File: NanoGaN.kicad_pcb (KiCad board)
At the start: 6 copper layers, 54 x 94 mm, 222 parts, among them J1 U_DC, J10 Conn_01x06, J11 Conn_01x04, J12 USB4085-GF-A, J14 Conn_01x03, J2 GND, J3 Phase_U, J4 Phase_V, J5 Phase_W, J6 FTSH-107-01-L-DV-K-TR, J7 Conn_01x03, J8 Conn_01x02, J9 Conn_01x07, Q1 IGC025S08S1, Q2 IGC025S08S1, Q3 IGC025S08S1, Q4 IGC025S08S1, Q5 IGC025S08S1, Q6 IGC025S08S1, Q7 Si2302CDS, U1 STM32H723VGTx, U10 SN74LVC1G66DCKR, U11 SN74LVC1G66DCKR, U12 LMG1205YFXR, U13 BMI323, U14 AS5047P-ATST, U15 TCAN1044VDRQ1, U16 SN74LVC1G66DCKR, U17 AD8418, U18 SN74LVC1G66DCKR, U19 NCS2220AMUT1G, U2 LMR51635XDDCR, U20 NCS2220AMUT1G, U21 NCS2220AMUT1G, U3 AMS1117, U4 AD8418, U5 LMG1205YFXR, U6 SN74LVC1G66DCKR, U7 SN74LVC1G66DCKR, U8 LMG1205YFXR, U9 AD8418, X1 8MHz

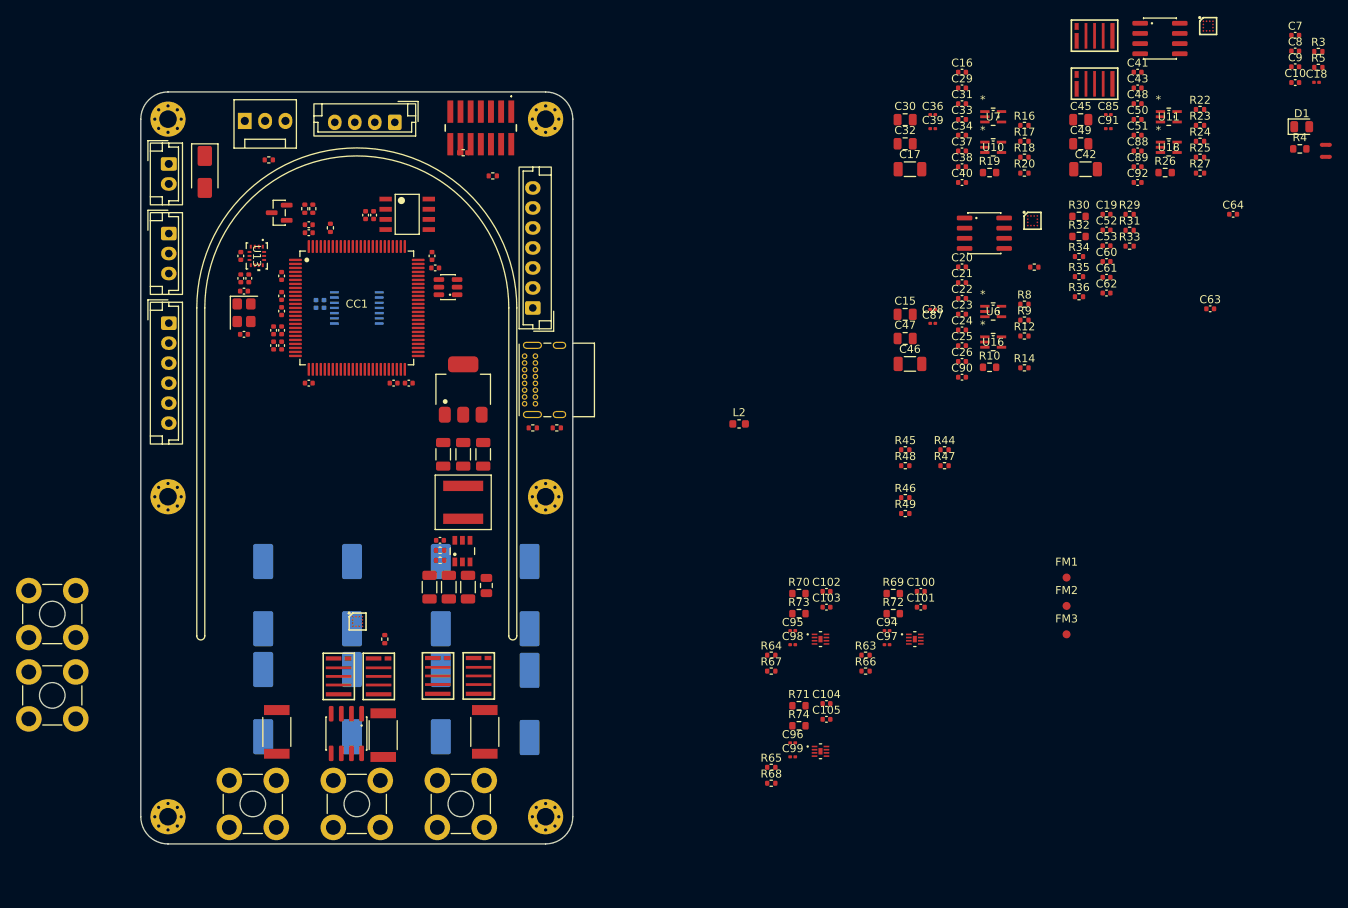
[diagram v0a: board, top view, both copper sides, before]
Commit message: added the first draft of the layout
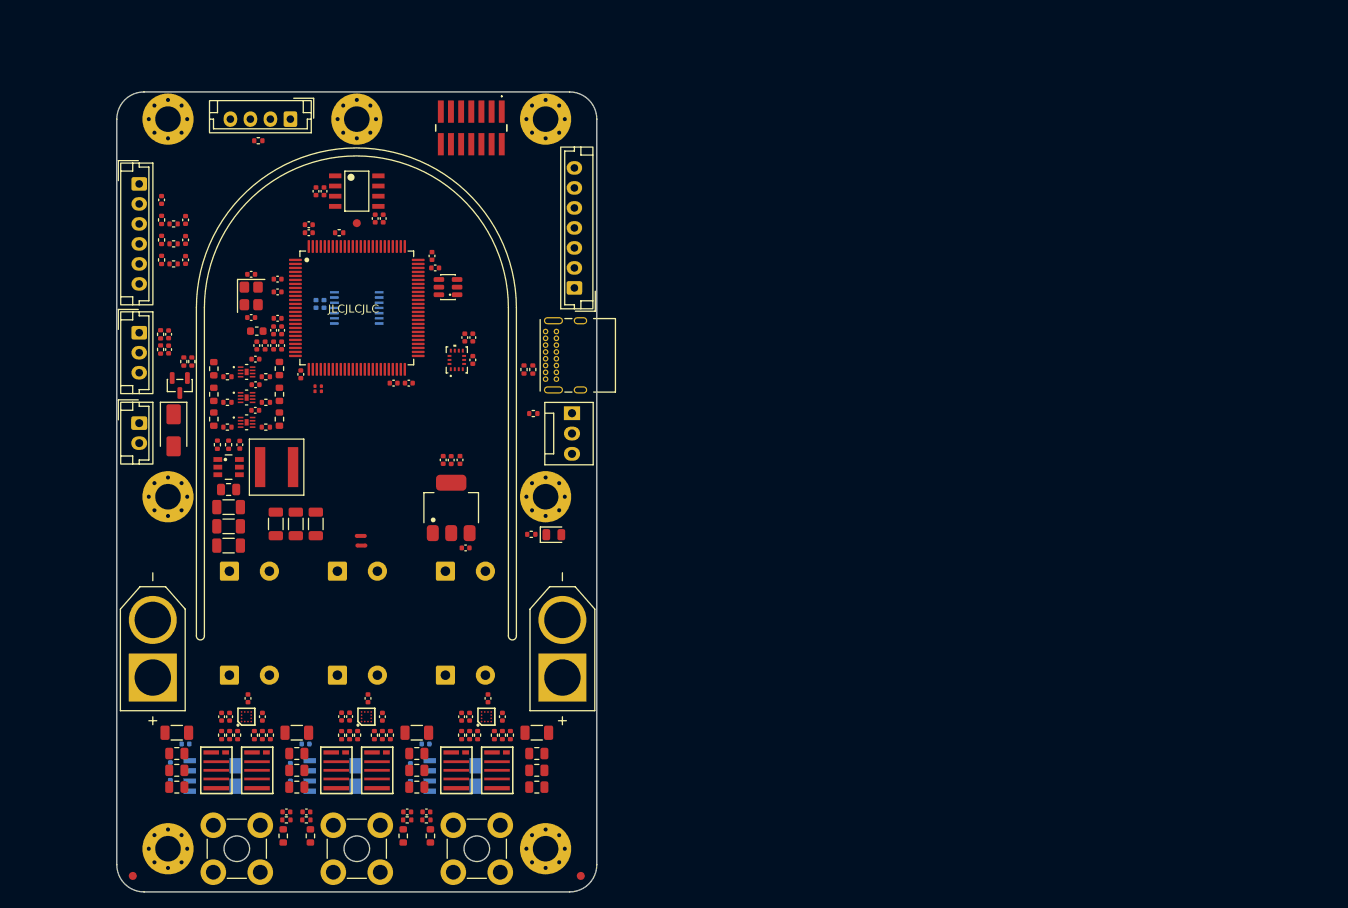
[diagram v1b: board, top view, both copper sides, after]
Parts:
- removed C102, C104: 1u, Capacitor_SMD:C_0402_1005Metric
- removed C103, C105: 100n, Capacitor_SMD:C_0402_1005Metric
- removed C96, C97, C98, C99: 1n, Capacitor_SMD:C_0201_0603Metric
- removed R28: 1m, NanoGaN:RES_00FEA_VIS-L
- removed R30, R32: 10k, Resistor_SMD:R_0603_1608Metric
- removed R7: 10k, Resistor_SMD:R_0402_1005Metric
- removed U10, U11, U16, U18: SN74LVC1G66DCKR, NanoGaN:DCK5
- removed U17, U9: AD8418, Package_SO:SOIC-8_3.9x4.9mm_P1.27mm
- added C67: 100n, Capacitor_SMD:C_0805_2012Metric, F.Cu at (152.7, 134.9)
- added C68: 1u, Capacitor_SMD:C_1206_3216Metric, F.Cu at (167.7, 128.1)
- added MH7: M3, MountingHole:MountingHole_3.2mm_M3_Pad_Via, F.Cu at (168.8, 142.6)
- C100: value 1u -> 100n
- C11, C12, C13, C14, C27, C35: value 150u -> 470u; footprint Capacitor_SMD:CP_Elec_10x10.5 -> Capacitor_THT:CP_Radial_D12.5mm_P5.00mm
- C18, C36, C85, C87: footprint Capacitor_SMD:C_0201_0603Metric -> Capacitor_SMD:C_0402_1005Metric
- C24, C25, C33, C38, C89: moved to B.Cu
- C26: value 1u -> 100n; moved to B.Cu
- C28, C39, C91: value 1n -> 100p; footprint Capacitor_SMD:C_0201_0603Metric -> Capacitor_SMD:C_0402_1005Metric; moved to B.Cu
- C37: value 1u -> 4u7
- C40: value 15n -> 4u7
- C44, C81: value 150u -> 100n; footprint Capacitor_SMD:CP_Elec_10x10.5 -> Capacitor_SMD:C_0805_2012Metric; moved to F.Cu
- C50: footprint Capacitor_SMD:C_0402_1005Metric -> Capacitor_SMD:C_0805_2012Metric
- C88: value 1u -> 100n; footprint Capacitor_SMD:C_0402_1005Metric -> Capacitor_SMD:C_0805_2012Metric
- C90: value 15n -> 100n; footprint Capacitor_SMD:C_0402_1005Metric -> Capacitor_SMD:C_0805_2012Metric
- C92: value 15n -> 100n
- J1: value U_DC -> XT60-M; footprint TerminalBlock_Wuerth:Wuerth_REDCUBE-THR_WP-THRBU_74650073_THR -> NanoGaN:AMASS_XT60-M
- J2: value GND -> XT60-M; footprint TerminalBlock_Wuerth:Wuerth_REDCUBE-THR_WP-THRBU_74650073_THR -> NanoGaN:AMASS_XT60-M
- MH1, MH2, MH3, MH4, MH5, MH6: value M2 -> M3; footprint MountingHole:MountingHole_2.2mm_M2_Pad_Via -> MountingHole:MountingHole_3.2mm_M3_Pad_Via
- R11, R21: value 1m -> 10k; footprint NanoGaN:RES_00FEA_VIS-L -> Resistor_SMD:R_0402_1005Metric
- U4: value AD8418 -> ACS37030LLZATR-065B3; footprint Package_SO:SOIC-8_3.9x4.9mm_P1.27mm -> NanoGaN:ACS37030LLZATR020B3; moved to B.Cu
- U6, U7: value SN74LVC1G66DCKR -> ACS37030LLZATR-065B3; footprint NanoGaN:DCK5 -> NanoGaN:ACS37030LLZATR020B3; moved to B.Cu
- moved U12 148.0 mm to (131.4, 126.1), turned to 90 degrees
- moved R5 147.7 mm to (151.5, 139.0)
- moved C18 145.7 mm to (151.5, 138.0)
- moved R23 143.3 mm to (129.3, 128.4), turned to -90 degrees
- moved C91 141.8 mm to (121.9, 132.3), turned to 90 degrees
- moved R4 141.2 mm to (151.0, 141.0), turned to 90 degrees
- moved R25 140.3 mm to (130.3, 128.4), turned to 90 degrees
- moved R22 140.1 mm to (134.4, 128.4), turned to -90 degrees
- moved C41 140.0 mm to (128.3, 126.1), turned to -90 degrees
- moved R27 139.9 mm to (136.4, 139.0)
- moved R24 139.6 mm to (132.4, 128.4), turned to 90 degrees
- moved Q6 139.3 mm to (127.9, 132.8), turned to -90 degrees
- moved Q5 139.2 mm to (133.0, 132.8), turned to -90 degrees
- moved C89 139.2 mm to (123.7, 129.5), turned to 180 degrees
- moved C43 138.1 mm to (129.3, 126.1), turned to -90 degrees
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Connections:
- net /MCU/BOOT0 renamed BOOT0
- C100 pad 1: +3V3A -> +3V3
- C101 pad 1: +3V3A -> +3V3
- C24 pad 1: +3V3A -> +3V3
- C24 pad 2: AGND -> PGND
- C25 pad 1: Net-(U16-A) -> /HalfBridgeU/I_CURR_SENS-
- C25 pad 2: /HalfBridgeU/U_PHASE_SENS -> PGND
- C26 pad 1: +3V3A -> /HalfBridgeV/I_CURR_SENS-
- C26 pad 2: AGND -> PGND
- C28 pad 1: /HalfBridgeU/I_CURR_SENS -> /HalfBridgeU/I_CURR_SENS+
- C28 pad 2: AGND -> PGND
- C33 pad 1: Net-(U7-A) -> /HalfBridgeW/I_CURR_SENS-
- C33 pad 2: /HalfBridgeV/U_PHASE_SENS -> PGND
- C37 pad 1: +3V3A -> +3V3
- C37 pad 2: AGND -> GND
- C38 pad 1: +3V3A -> +3V3
- C38 pad 2: AGND -> PGND
- C39 pad 1: /HalfBridgeV/I_CURR_SENS -> /HalfBridgeV/I_CURR_SENS+
- C39 pad 2: AGND -> PGND
- C40 pad 1: /HalfBridgeV/I_CURR_SENS -> +3V3
- C40 pad 2: Net-(U10-A) -> GND
- C50 pad 1: Net-(U11-A) -> U_DC
- C50 pad 2: /HalfBridgeW/U_PHASE_SENS -> PGND
- C88 pad 1: +3V3A -> U_DC
- C88 pad 2: AGND -> PGND
- C89 pad 1: +3V3A -> +3V3
- C89 pad 2: AGND -> PGND
- C90 pad 1: /HalfBridgeU/I_CURR_SENS -> U_DC
- C90 pad 2: Net-(U6-A) -> PGND
- C91 pad 1: /HalfBridgeW/I_CURR_SENS -> /HalfBridgeW/I_CURR_SENS+
- C91 pad 2: AGND -> PGND
- C92 pad 1: /HalfBridgeW/I_CURR_SENS -> +3V3
- C92 pad 2: Net-(U18-A) -> AGND
- C95 pad 1: /HalfBridgeU/DAC_OCP_P -> /HalfBridgeU/DAC_OCP_N
- MH3 pad 1: PGND -> GND
- R11 pad 1: /HalfBridgeU/HS -> /Connectors/EXT_TEMP2
- R11 pad 2: /HalfBridgeU/PHASE -> GND
- R21 pad 1: /HalfBridgeV/HS -> /Connectors/EXT_TEMP1
- R21 pad 2: /HalfBridgeV/PHASE -> GND
- U1 pad 22: unconnected-(U1-PA0-Pad22) -> /HalfBridgeU/U_PHASE_SENS
- U1 pad 23: unconnected-(U1-PA1-Pad23) -> /HalfBridgeV/U_PHASE_SENS
- U1 pad 24: unconnected-(U1-PA2-Pad24) -> /HalfBridgeW/U_PHASE_SENS
- U1 pad 30: /HalfBridgeW/I_CURR_SENS -> /HalfBridgeU/I_CURR_SENS+
- U1 pad 31: /HalfBridgeW/U_PHASE_SENS -> /HalfBridgeU/I_CURR_SENS-
- U1 pad 32: /HalfBridgeV/U_PHASE_SENS -> /HalfBridgeV/I_CURR_SENS+
- U1 pad 33: /HalfBridgeV/I_CURR_SENS -> /HalfBridgeV/I_CURR_SENS-
- U1 pad 34: /HalfBridgeU/I_CURR_SENS -> /HalfBridgeW/I_CURR_SENS-
- U1 pad 35: /HalfBridgeU/U_PHASE_SENS -> /HalfBridgeW/I_CURR_SENS+
- U1 pad 37: /HalfBridgeU/EN_FILTER_I -> unconnected-(U1-PE7-Pad37)
- U1 pad 7: unconnected-(U1-PC13-Pad7) -> /Connectors/HALL1
- U1 pad 8: unconnected-(U1-PC14-Pad8) -> /Connectors/HALL2
- U1 pad 81: FDCAN1_RX -> /MCU/UART4_RX
- U1 pad 82: FDCAN1_TX -> /MCU/UART4_TX
- U1 pad 83: FDCAN1_STB -> unconnected-(U1-PD2-Pad83)
- U1 pad 85: unconnected-(U1-PD4-Pad85) -> FDCAN1_STB
- U1 pad 9: unconnected-(U1-PC15-Pad9) -> /Connectors/HALL3
- U1 pad 90: /Connectors/SERVO -> unconnected-(U1-PB4(NJTRST)-Pad90)
- U1 pad 91: /Connectors/SERVO -> unconnected-(U1-PB5-Pad91)
- U1 pad 92: /Connectors/VCP_RX -> unconnected-(U1-PB6-Pad92)
- U1 pad 93: /Connectors/VCP_TX -> unconnected-(U1-PB7-Pad93)
- U1 pad 95: unconnected-(U1-PB8-Pad95) -> FDCAN1_RX
- U1 pad 96: /Connectors/FAN_PWM -> FDCAN1_TX
- U13 pad 1: SPI4_MISO -> SPI2_MISO
- U13 pad 12: SPI4_NSS -> SPI2_NSS
- U13 pad 13: SPI4_SCK -> SPI2_SCK
- U13 pad 14: SPI4_MOSI -> SPI2_MOSI
- U14 pad 1: SPI2_NSS -> SPI4_NSS
- U14 pad 2: SPI2_SCK -> SPI4_SCK
- U14 pad 3: SPI2_MISO -> SPI4_MISO
- U14 pad 4: SPI2_MOSI -> SPI4_MOSI
- U19 pad 2: /HalfBridgeU/I_CURR_SENS -> /HalfBridgeU/I_CURR_SENS+
- U19 pad 6: /HalfBridgeU/I_CURR_SENS -> /HalfBridgeU/I_CURR_SENS+
- U19 pad 8: +3V3A -> +3V3
- U20 pad 2: /HalfBridgeV/I_CURR_SENS -> /HalfBridgeV/I_CURR_SENS+
- U20 pad 6: /HalfBridgeV/I_CURR_SENS -> /HalfBridgeV/I_CURR_SENS+
- U20 pad 8: +3V3A -> +3V3
- U21 pad 2: /HalfBridgeW/I_CURR_SENS -> /HalfBridgeW/I_CURR_SENS+
- U21 pad 6: /HalfBridgeW/I_CURR_SENS -> /HalfBridgeW/I_CURR_SENS+
- U21 pad 8: +3V3A -> +3V3
- U4 pad 1: /HalfBridgeU/PHASE -> /HalfBridgeU/HS
- U4 pad 2: AGND -> /HalfBridgeU/PHASE
- U4 pad 3: AGND -> PGND
- U4 pad 4: unconnected-(U4-NC-Pad4) -> /HalfBridgeU/I_CURR_SENS-
- U4 pad 5: /HalfBridgeU/I_CURR_SENS -> /HalfBridgeU/I_CURR_SENS+
- U4 pad 6: +3V3A -> +3V3
- U6 pad 1: Net-(U6-A) -> /HalfBridgeV/HS
- U6 pad 2: AGND -> /HalfBridgeV/PHASE
- U6 pad 4: /HalfBridgeU/EN_FILTER_I -> /HalfBridgeV/I_CURR_SENS-
- U6 pad 5: +3V3A -> /HalfBridgeV/I_CURR_SENS+
- U7 pad 1: Net-(U7-A) -> /HalfBridgeW/HS
- U7 pad 2: PGND -> /HalfBridgeW/PHASE
- U7 pad 4: /HalfBridgeU/EN_FILTER_U -> /HalfBridgeW/I_CURR_SENS-
- U7 pad 5: +3V3A -> /HalfBridgeW/I_CURR_SENS+
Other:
- board size 54 x 94 mm -> 60 x 100 mm
- board text added: "JLCJLCJLC"
